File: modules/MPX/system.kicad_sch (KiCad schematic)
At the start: 2 parts, among them J1 CardConnector

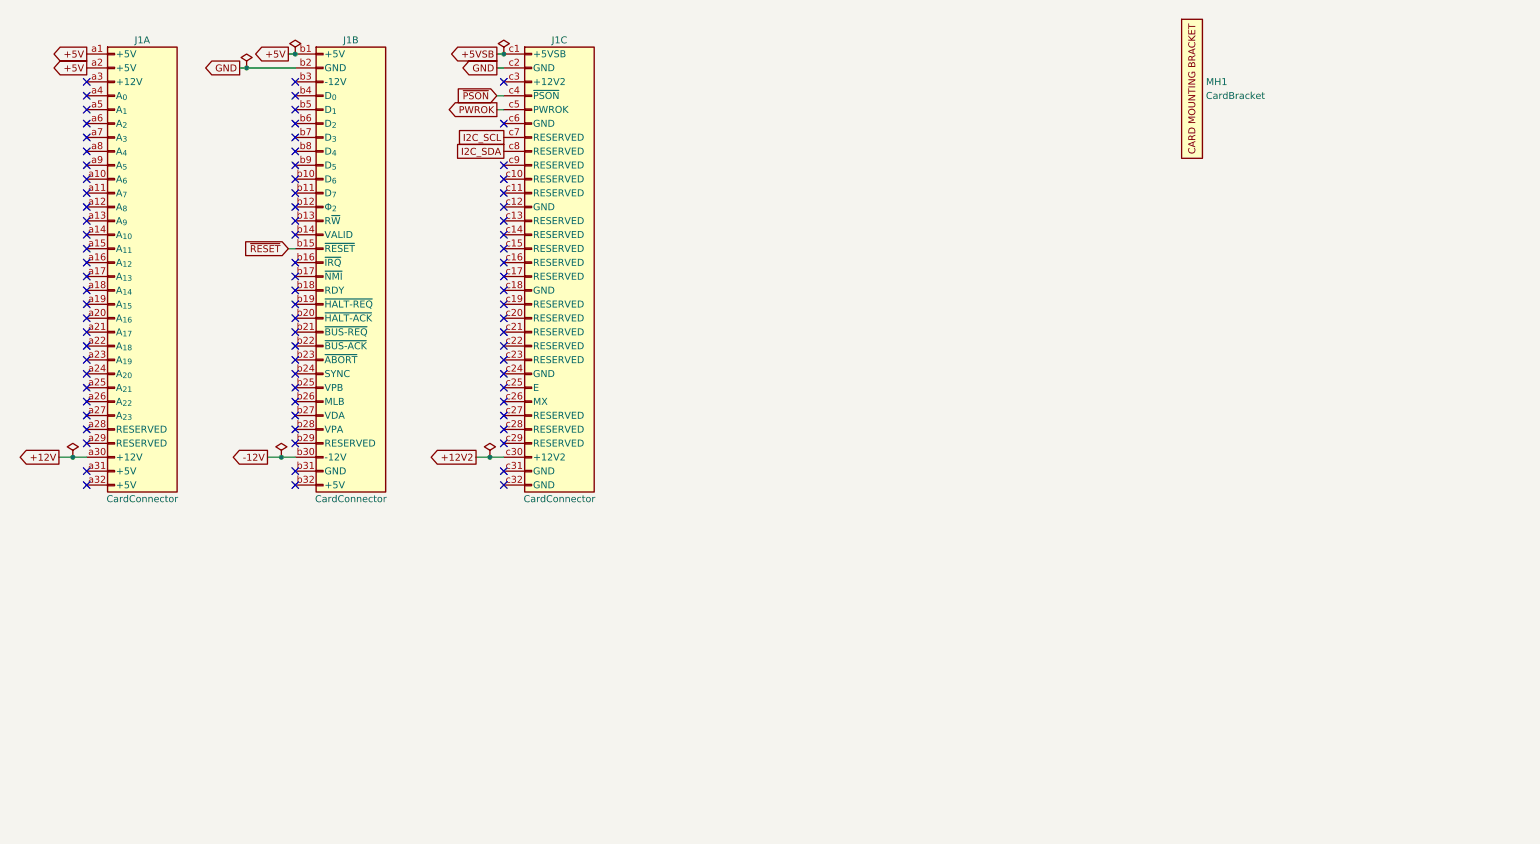
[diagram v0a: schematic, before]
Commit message: minor PW PCB tweaks
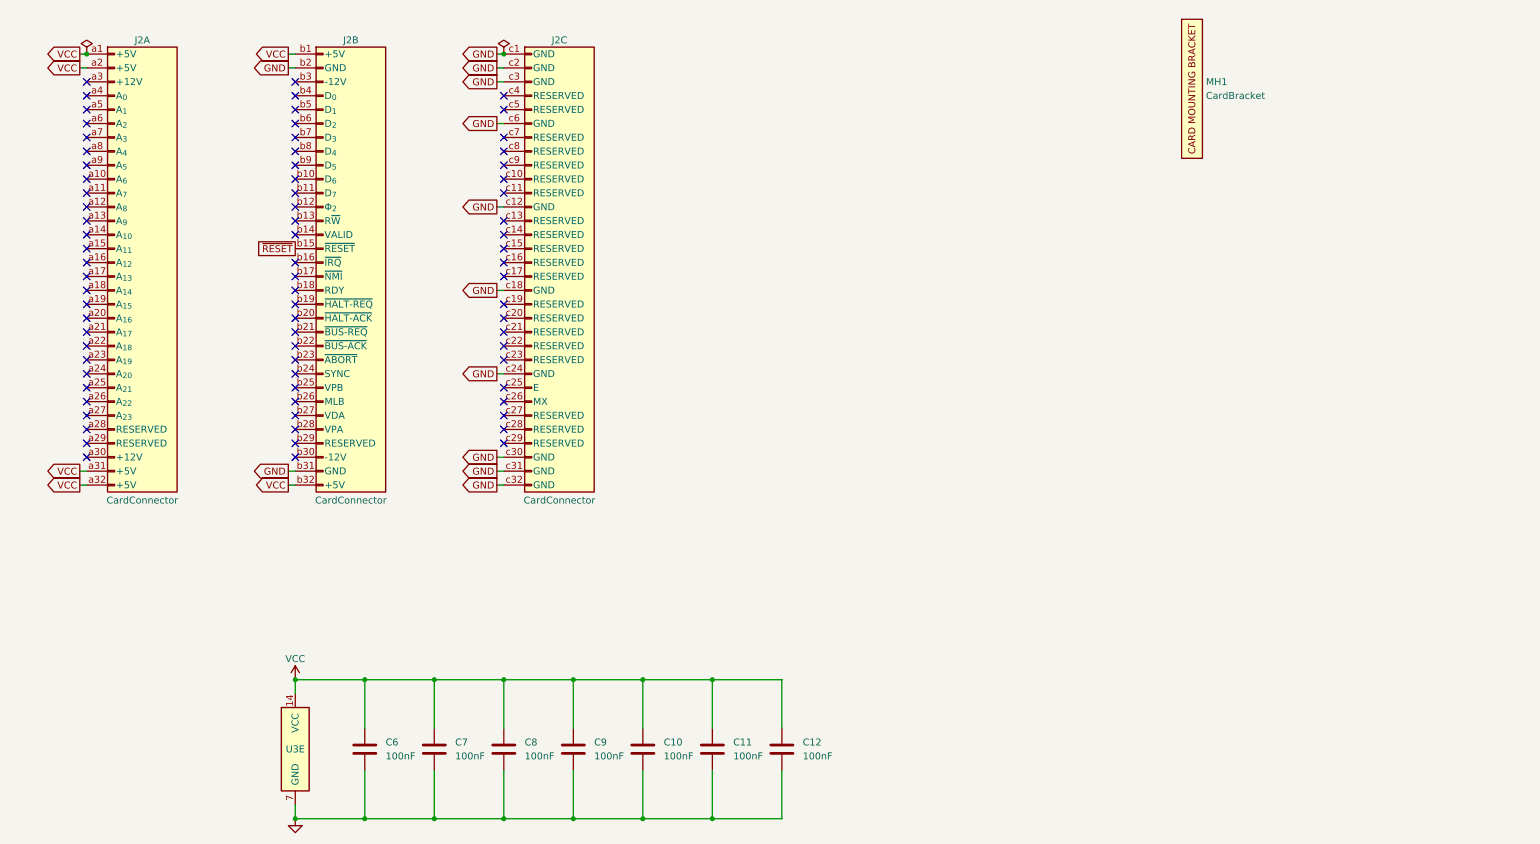
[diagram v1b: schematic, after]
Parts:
- added C10, C11, C12, C6, C7, C8, C9: 100nF, IMNOTWOPR:C_Rect_P200mil, symbol IMNOTWOPR:C
- added U3: 74NC00, IMNOTWOPR:DIP-14N, symbol IMNOTWOPR:7400
- renumbered J1 to J2
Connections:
- net +12V2 is gone; now on net GND: J2.c30 (GND)
- net +5V is gone; now on net VCC: J2.a1 (+5V), J2.a2 (+5V), J2.b1 (+5V)
- net +5VSB is gone; now on net GND: J2.c1 (GND)
- net GND: now also J2.b31 (GND), J2.c12 (GND), J2.c18 (GND), J2.c24 (GND), J2.c3 (GND), J2.c31 (GND), J2.c32 (GND), J2.c6 (GND), C10.2, C11.2, C12.2, C6.2, C7.2, C8.2, C9.2, U3.7 (GND)
- net VCC: now reaches J2.b32 (+5V)
- net VCC: now also J2.a31 (+5V), J2.a32 (+5V), C10.1, C11.1, C12.1, C6.1, C7.1, C8.1, C9.1, U3.14 (VCC)
- net +12V: no longer names the net of J2.a30 (+12V)
- net -12V: no longer names the net of J2.b30 (-12V)
- net I2C_SCL: no longer names the net of J2.c7 (RESERVED)
- net I2C_SDA: no longer names the net of J2.c8 (RESERVED)
- net PWROK: no longer names the net of J2.c5 (RESERVED)
- net ~{PSON}: no longer names the net of J2.c4 (RESERVED)
- no-connect marks 82 -> 77
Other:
- title: PWR -> MPU-65X

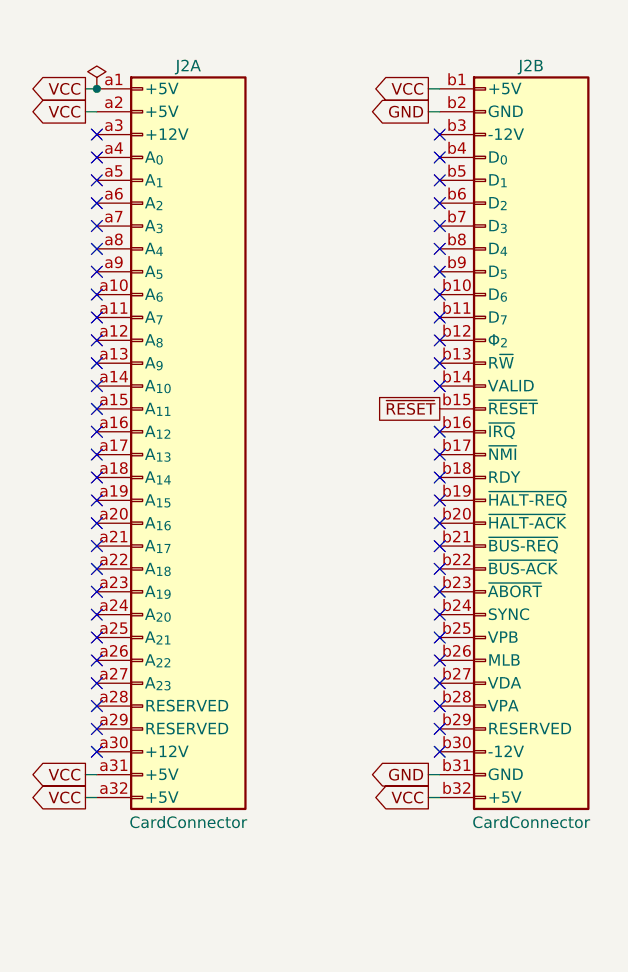
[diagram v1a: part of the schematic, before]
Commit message: project cleanup
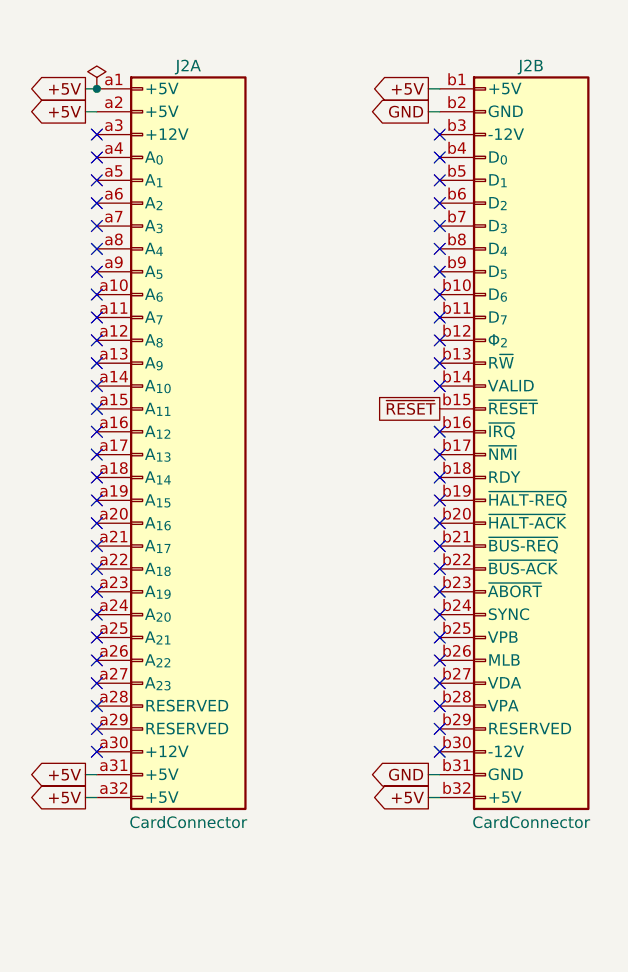
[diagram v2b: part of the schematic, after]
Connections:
- net VCC: no longer J2.a1 (+5V), J2.a2 (+5V), J2.a31 (+5V), J2.a32 (+5V), J2.b1 (+5V), J2.b32 (+5V)
- new net +5V: J2.a1 (+5V), J2.a2 (+5V), J2.a31 (+5V), J2.a32 (+5V), J2.b1 (+5V), J2.b32 (+5V)
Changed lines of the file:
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@@
 		)
 	)
-	(global_label "VCC"
+	(global_label "+5V"
 		(shape output)
 		(at 24.13 104.14 180)
@@
 		)
 		(property "Intersheetrefs" "${INTERSHEET_REFS}"
-			(at 17.5162 104.14 0)
+			(at 17.1792 104.14 0)
 			(hide yes)
 			(show_name no)
@@
 		)
 	)
-	(global_label "VCC"
+	(global_label "+5V"
 		(shape output)
 		(at 62.23 25.4 180)
@@
 		)
 		(property "Intersheetrefs" "${INTERSHEET_REFS}"
-			(at 55.6162 25.4 0)
+			(at 55.2792 25.4 0)
 			(hide yes)
 			(show_name no)
@@
 		)
 	)
-	(global_label "VCC"
+	(global_label "+5V"
 		(shape output)
 		(at 24.13 25.4 180)
@@
 		)
 		(property "Intersheetrefs" "${INTERSHEET_REFS}"
-			(at 17.5162 25.4 0)
-			(hide yes)
-			(show_name no)
-			(do_not_autoplace no)
-			(effects
-				(font
-					(size 1.27 1.27)
-				)
-				(justify right)
-			)
-		)
-	)
-	(global_label "VCC"
+			(at 17.1792 25.4 0)
+			(hide yes)
+			(show_name no)
+			(do_not_autoplace no)
+			(effects
+				(font
+					(size 1.27 1.27)
+				)
+				(justify right)
+			)
+		)
+	)
+	(global_label "+5V"
 		(shape output)
 		(at 24.13 101.6 180)
@@
 		)
 		(property "Intersheetrefs" "${INTERSHEET_REFS}"
-			(at 17.5162 101.6 0)
+			(at 17.1792 101.6 0)
 			(hide yes)
 			(show_name no)
@@
 		)
 	)
-	(global_label "VCC"
+	(global_label "+5V"
 		(shape output)
 		(at 62.23 104.14 180)
@@
 		)
 		(property "Intersheetrefs" "${INTERSHEET_REFS}"
-			(at 55.6162 104.14 0)
+			(at 55.2792 104.14 0)
 			(hide yes)
 			(show_name no)
@@
 		)
 	)
-	(global_label "VCC"
+	(global_label "+5V"
 		(shape output)
 		(at 24.13 27.94 180)
@@
 		)
 		(property "Intersheetrefs" "${INTERSHEET_REFS}"
-			(at 17.5162 27.94 0)
-			(hide yes)
-			(show_name no)
+			(at 17.1792 27.94 0)
+			(hide yes)
+			(show_name no)

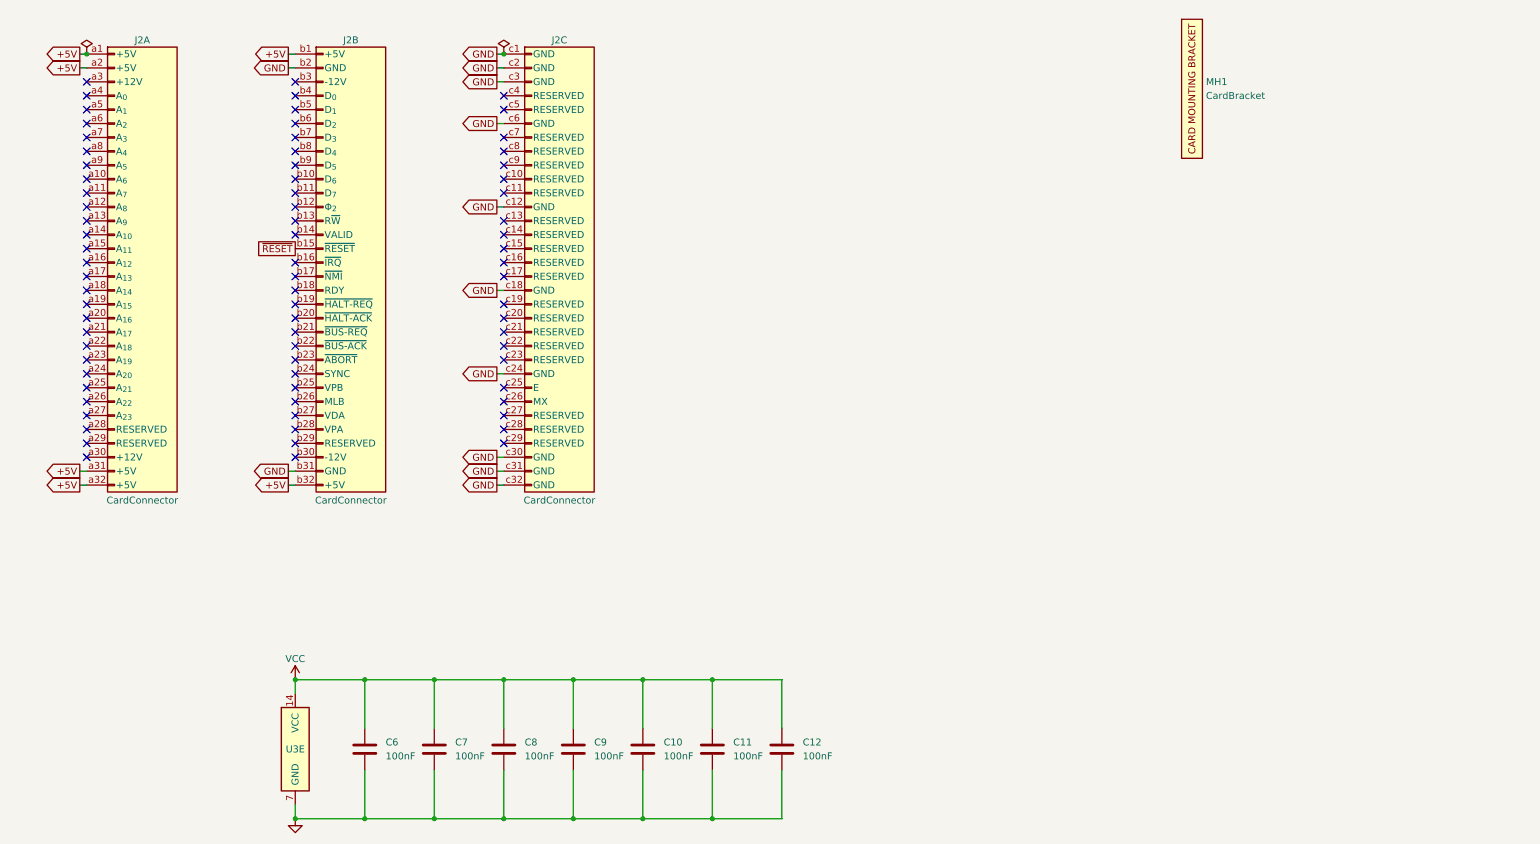
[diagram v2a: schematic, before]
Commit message: work on mpx module
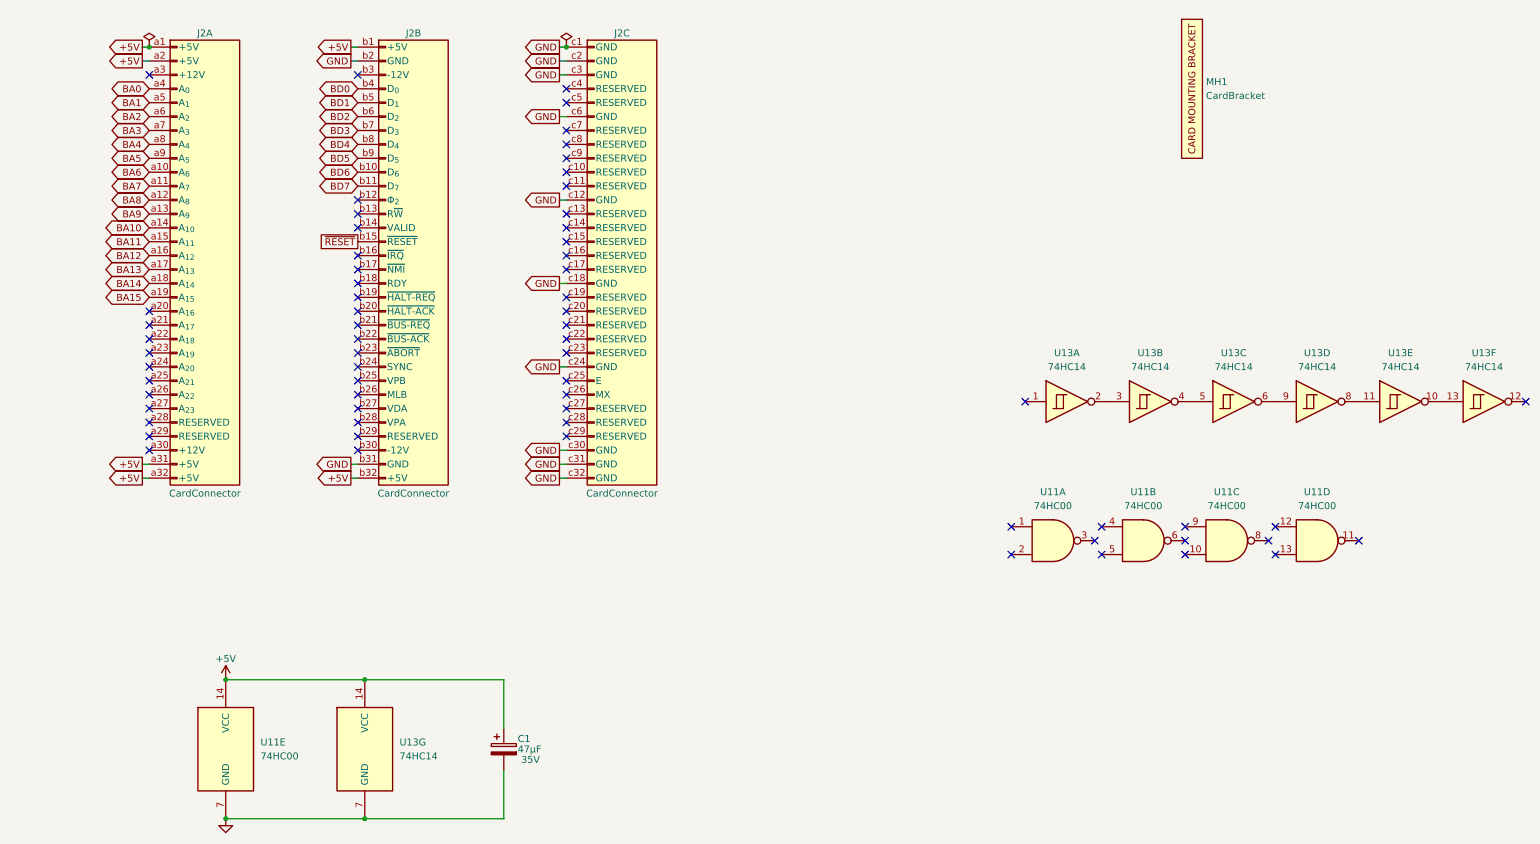
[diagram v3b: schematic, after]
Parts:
- removed C10, C11, C12, C6, C7, C8, C9: 100nF, IMNOTWOPR:C_Rect_P200mil, symbol IMNOTWOPR:C
- removed U3: 74NC00, IMNOTWOPR:DIP-14N, symbol IMNOTWOPR:7400
- added C1: 47µF, IMNOTWOPR:CP_Radial_Tantal_P100mil, symbol IMNOTWOPR:C_Polarized
- added U11: 74HC00, IMNOTWOPR:DIP-14N, symbol 74xx:74HC00
- added U13: 74HC14, IMNOTWOPR:DIP-14N, symbol 74xx:74HC14
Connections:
- net +5V: now also C1.1, U11.14 (VCC), U13.14 (VCC)
- net GND: now also C1.2, U11.7 (GND), U13.7 (GND)
- net BD6: now reaches J2.b10 (D_{6})
- net BD7: now reaches J2.b11 (D_{7})
- net BD0: now reaches J2.b4 (D_{0})
- net BD1: now reaches J2.b5 (D_{1})
- net BD2: now reaches J2.b6 (D_{2})
- net BD3: now reaches J2.b7 (D_{3})
- net BD4: now reaches J2.b8 (D_{4})
- net BD5: now reaches J2.b9 (D_{5})
- net BA6: now reaches J2.a10 (A_{6})
- net BA7: now reaches J2.a11 (A_{7})
- net BA8: now reaches J2.a12 (A_{8})
- net BA9: now reaches J2.a13 (A_{9})
- net BA10: now reaches J2.a14 (A_{10})
- net BA11: now reaches J2.a15 (A_{11})
- net BA12: now reaches J2.a16 (A_{12})
- net BA13: now reaches J2.a17 (A_{13})
- net BA14: now reaches J2.a18 (A_{14})
- net BA15: now reaches J2.a19 (A_{15})
- net BA0: now reaches J2.a4 (A_{0})
- net BA1: now reaches J2.a5 (A_{1})
- net BA2: now reaches J2.a6 (A_{2})
- net BA3: now reaches J2.a7 (A_{3})
- net BA4: now reaches J2.a8 (A_{4})
- net BA5: now reaches J2.a9 (A_{5})
- new net: U13.2, U13.3
- new net: U13.10, U13.13
- new net: U13.4, U13.5
- new net: U13.6, U13.9
- new net: U13.11, U13.8
- no-connect marks 77 -> 67
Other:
- title: MPU-65X -> MPX
- moved on the sheet: J2A, J2B, J2C

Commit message: cleanup and mpx work
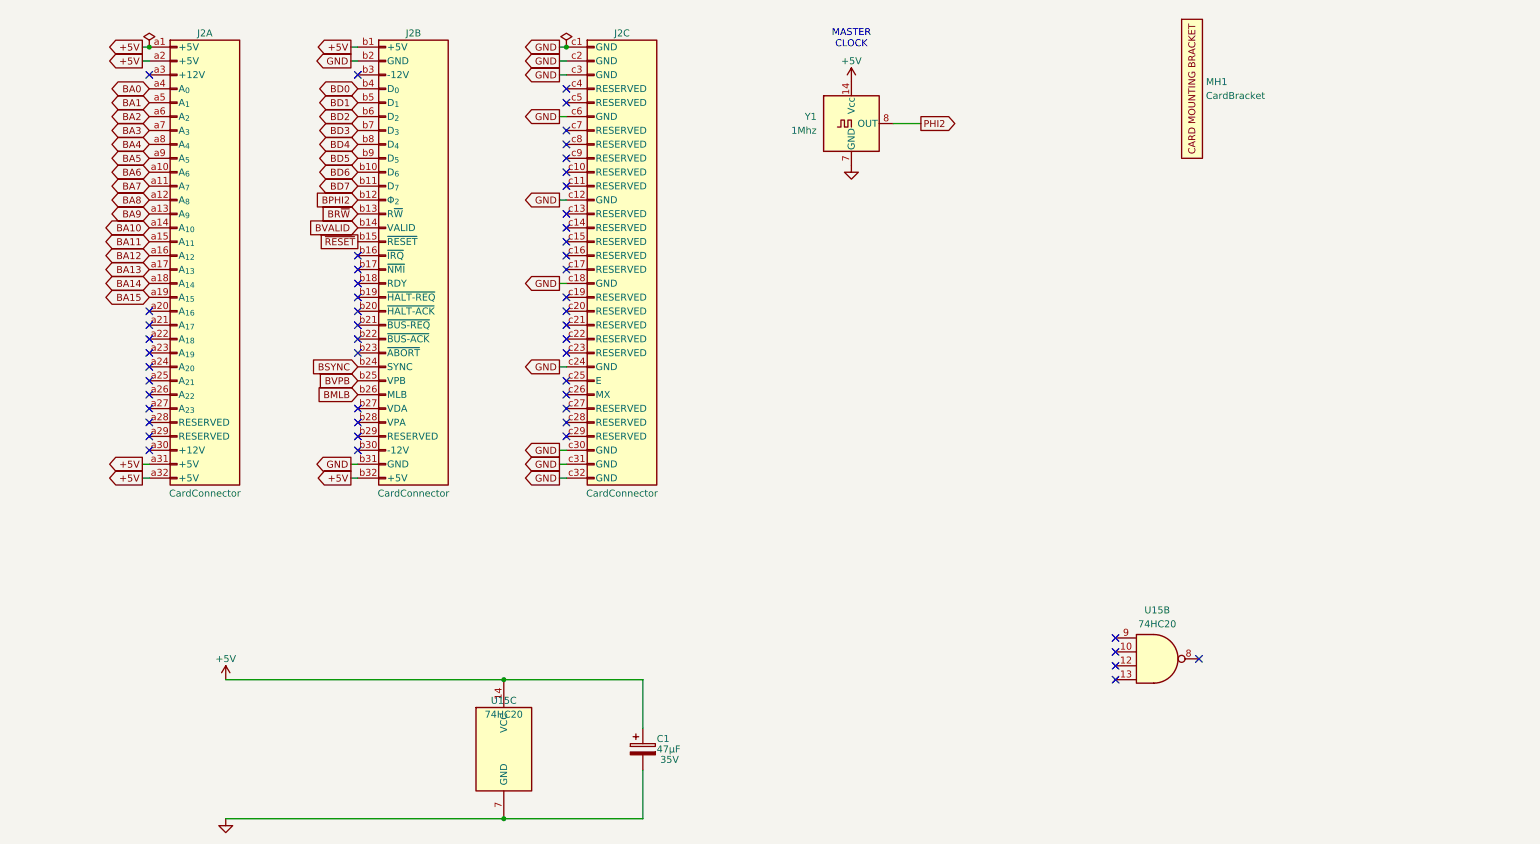
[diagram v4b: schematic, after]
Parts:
- removed U11: 74HC00, IMNOTWOPR:DIP-14N, symbol 74xx:74HC00
- removed U13: 74HC14, IMNOTWOPR:DIP-14N, symbol 74xx:74HC14
- added U15: 74HC20, IMNOTWOPR:DIP-14N, symbol 74xx:74LS20
- added Y1: 1Mhz, Oscillator:Oscillator_DIP-14, symbol Oscillator:ACO-xxxMHz
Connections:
- net +5V: now also U15.14 (VCC), Y1.14 (Vcc)
- net GND: now also U15.7 (GND), Y1.7 (GND)
- net BPHI2: now reaches J2.b12 (Φ_{2})
- net BR~{W}: now reaches J2.b13 (R~{W})
- net BVALID: now reaches J2.b14 (VALID)
- net BSYNC: now reaches J2.b24 (SYNC)
- net BVPB: now reaches J2.b25 (VPB)
- net BMLB: now reaches J2.b26 (MLB)
- new net PHI2: Y1.8 (OUT)
- no-connect marks 67 -> 52
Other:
- note added: "MASTER CLOCK"
- moved on the sheet: C1
